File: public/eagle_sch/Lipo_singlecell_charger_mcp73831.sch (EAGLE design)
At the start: 10 parts, among them U3 MCP73831, X1 USBSMD

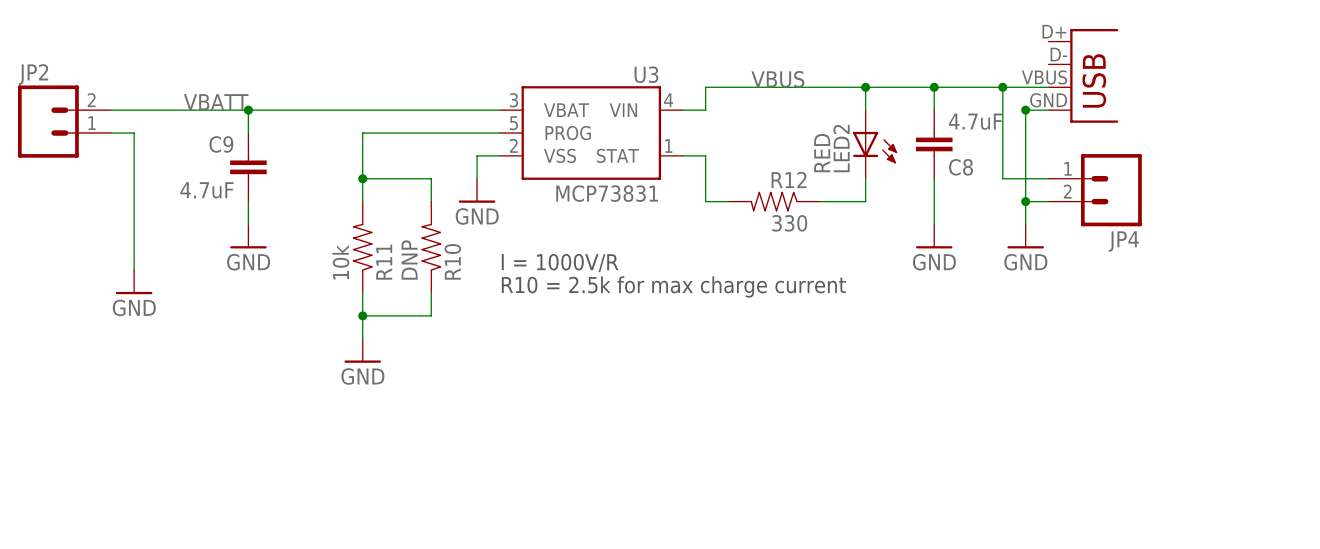
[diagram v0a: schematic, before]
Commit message: download sch
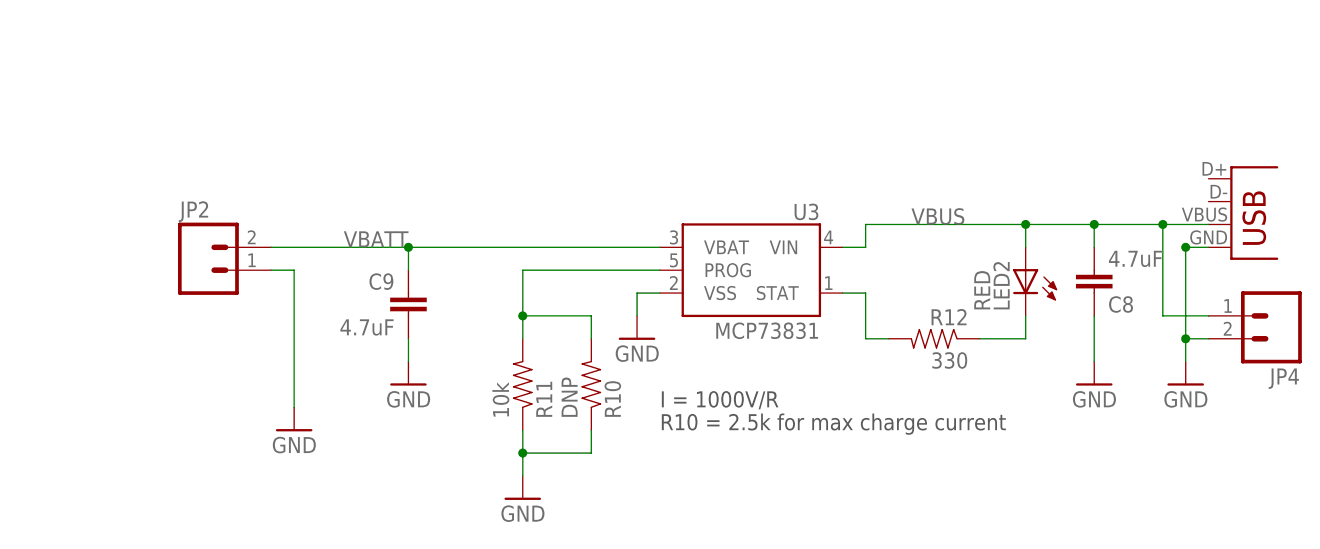
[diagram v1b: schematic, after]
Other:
- moved on the sheet: C8, C9, JP2, JP4, LED2, R10, R11, R12, U3
